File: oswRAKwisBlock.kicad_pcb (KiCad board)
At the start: 4 copper layers, 33.8 x 46 mm, 64 parts, among them J1 WisBlock, J2 0524352471, J4 10114830-10102LF, J5 USB micro, Q1 SI1308EDL-T1-GE3, U1 MCP73811T-420I/OT, U2 MAX2769B, U3 MAX8510EXK29+T, U4 MAX8510EXK29+T, Y1 TXETCDSANF-16.368000

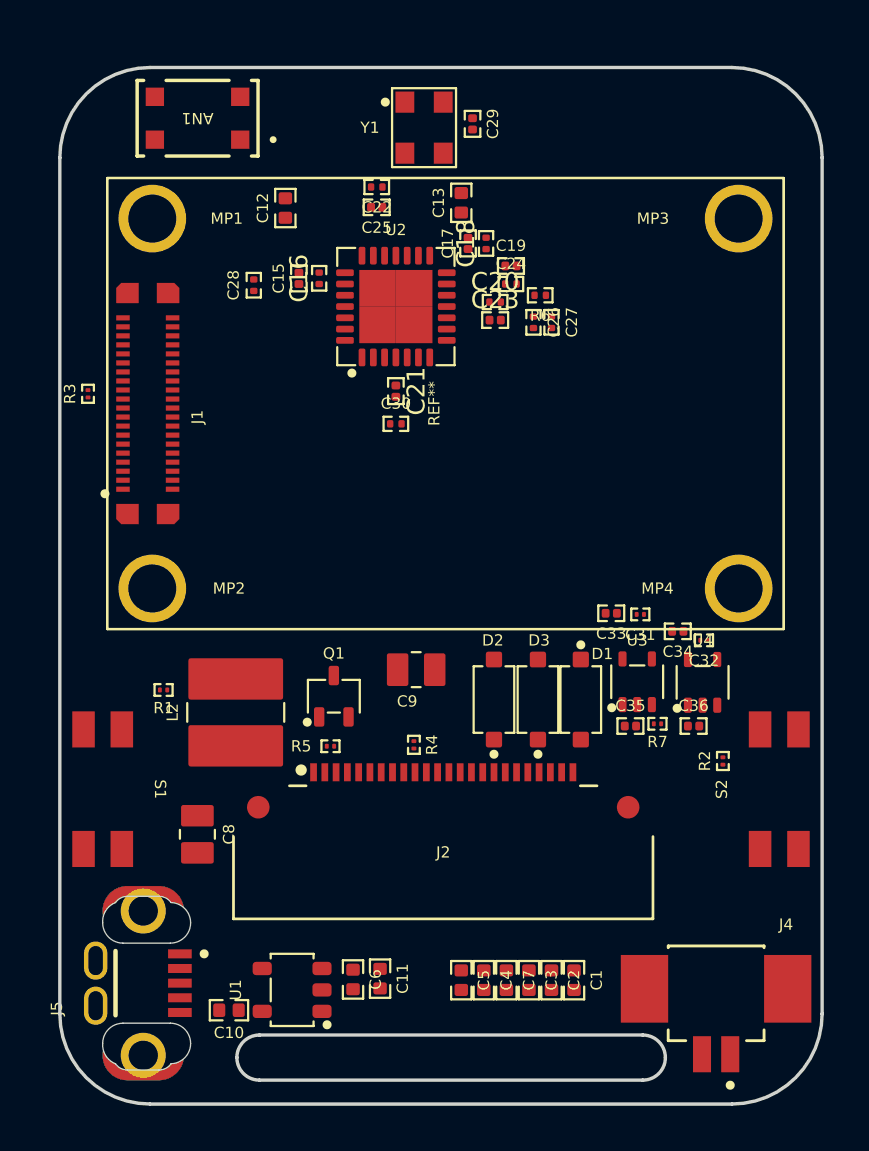
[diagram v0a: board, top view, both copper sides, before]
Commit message: starting to lay the board out.
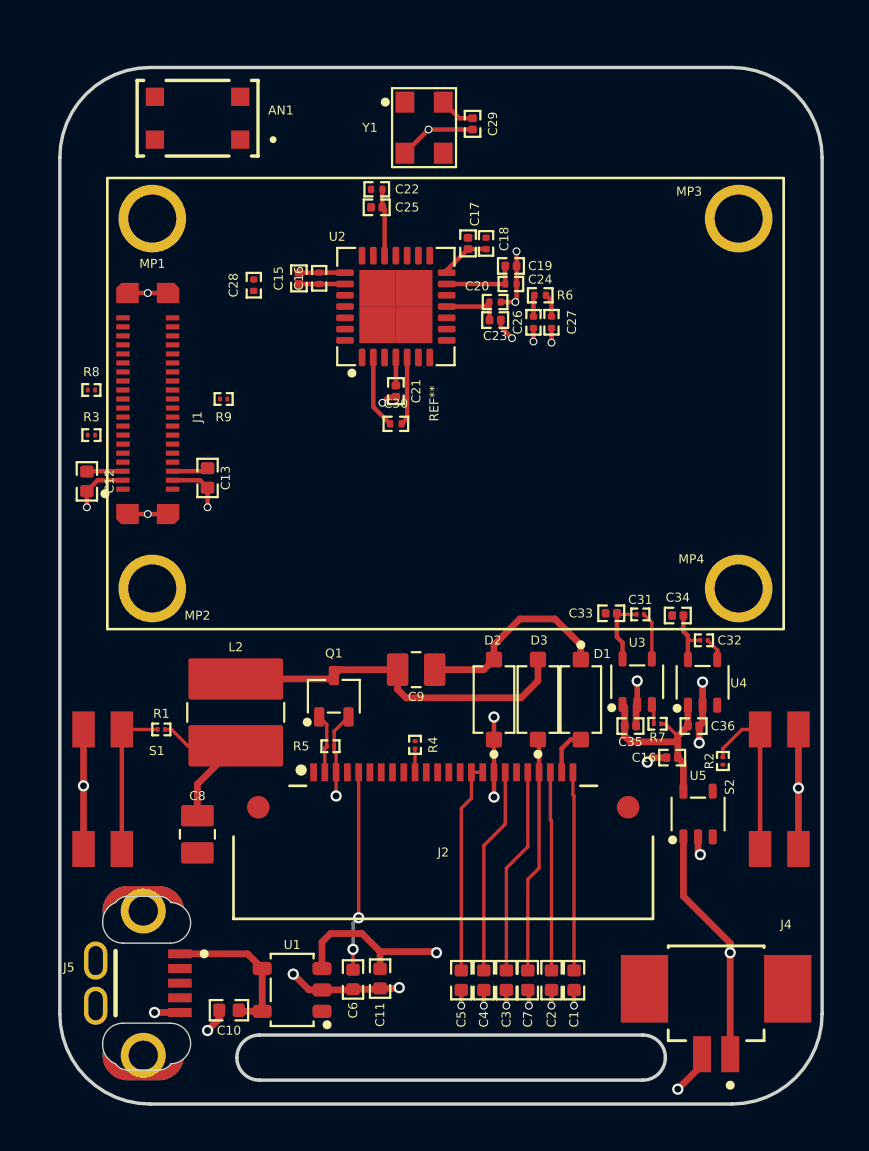
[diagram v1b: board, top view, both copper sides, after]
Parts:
- added C16: 1uF, AllardChip:CAPC60X30X39L17L, F.Cu at (147.0, 130.6)
- added R8: 10k, AllardChip:RESC40X20X15L10L, F.Cu at (121.2, 114.3)
- added R9: 10k, AllardChip:RESC40X20X15L10L, F.Cu at (127.1, 114.7)
- added U5: MIC5365-3.0YC5-TR, AllardSOT:SOT23-5P65_210X110L33X22L, F.Cu at (148.2, 133.1)
- moved C13 16.6 mm to (126.4, 118.2), turned to -90 degrees
- moved C12 15.0 mm to (121.0, 118.3), turned to -90 degrees
- moved R3 1.84 mm to (121.2, 116.3), turned to 0 degrees
- moved R1 1.75 mm to (124.3, 129.3)
- moved C3 1.00 mm to (139.7, 140.5)
- moved C7 0.95 mm to (140.6, 140.5)
- moved C34 0.70 mm to (147.2, 124.3)
- moved C22 0.10 mm to (133.9, 105.4)
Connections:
- J1 pad 22: unconnected-(J1-AIN1-Pad22) -> /~{GPS_PWR_SHDN}
- J1 pad 23: unconnected-(J1-BOOT-Pad23) -> Net-(J1-BOOT)
- J1 pad 24: unconnected-(J1-IO7-Pad24) -> /~{GPS_SHDN}
- J1 pad 25: unconnected-(J1-SPI_CS-Pad25) -> /SS
- J1 pad 26: unconnected-(J1-SPI_CLK-Pad26) -> /SCLK
- J1 pad 27: unconnected-(J1-SPI_MISO-Pad27) -> /GPS_MISO
- J1 pad 28: unconnected-(J1-SPI_MOSI-Pad28) -> /MOSI
- J1 pad 29: unconnected-(J1-IO1-Pad29) -> /BUSY
- J1 pad 30: unconnected-(J1-IO2-Pad30) -> /BTN1
- J1 pad 31: unconnected-(J1-IO3-Pad31) -> /RES
- J1 pad 32: unconnected-(J1-IO4-Pad32) -> /BTN2
- J1 pad 37: unconnected-(J1-IO5-Pad37) -> /~{GPS_IDLE}
- J1 pad 38: unconnected-(J1-IO6-Pad38) -> /~{GPS_CS}
- J1 pad FS3: (no net) -> GND
- R7 pad 2: /gpsMod/~{GPS_PWR_SHDN} -> /~{GPS_PWR_SHDN}
- U2 pad 10: /gpsMod/~{GPS_CS} -> /~{GPS_CS}
- U2 pad 24: /gpsMod/~{GPS_IDLE} -> /~{GPS_IDLE}
- U2 pad 7: /gpsMod/~{GPS_SHDN} -> /~{GPS_SHDN}
- U2 pad 8: /gpsMod/GPS_MISO -> /GPS_MISO
- U2 pad 9: /gpsMod/GPS_SCLK -> /SCLK
- U3 pad 3: /gpsMod/~{GPS_PWR_SHDN} -> /~{GPS_PWR_SHDN}
- U4 pad 3: /gpsMod/~{GPS_PWR_SHDN} -> /~{GPS_PWR_SHDN}
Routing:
- net GND: track 0.00 -> 58.0 mm, vias 0 -> 32
- net Net-(U1-V_{BAT}): track 0.00 -> 31.0 mm, vias 0 -> 2
- net VDD: track 0.00 -> 28.9 mm
- net Net-(Q1-D): track 0.00 -> 15.9 mm
- net VDD_GPS_A: track 0.00 -> 12.5 mm
- net /PREVGH: track 0.00 -> 10.5 mm
- net VDD_GPS_B: track 0.00 -> 9.71 mm
- net Net-(J2-Pin_20): track 0.00 -> 9.18 mm
- net Net-(J2-Pin_18): track 0.00 -> 9.18 mm
- net Net-(D1-K): track 0.00 -> 8.92 mm
- net Net-(J2-Pin_5): track 0.00 -> 8.86 mm, vias 0 -> 2
- net Net-(J2-Pin_24): track 0.00 -> 8.81 mm
- net Net-(J2-Pin_22): track 0.00 -> 8.81 mm
- net /BTN2: track 0.00 -> 7.69 mm
- net /BTN1: track 0.00 -> 6.89 mm
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- added copper zone on In1.Cu, net GND

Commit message: Moving some stuff around.
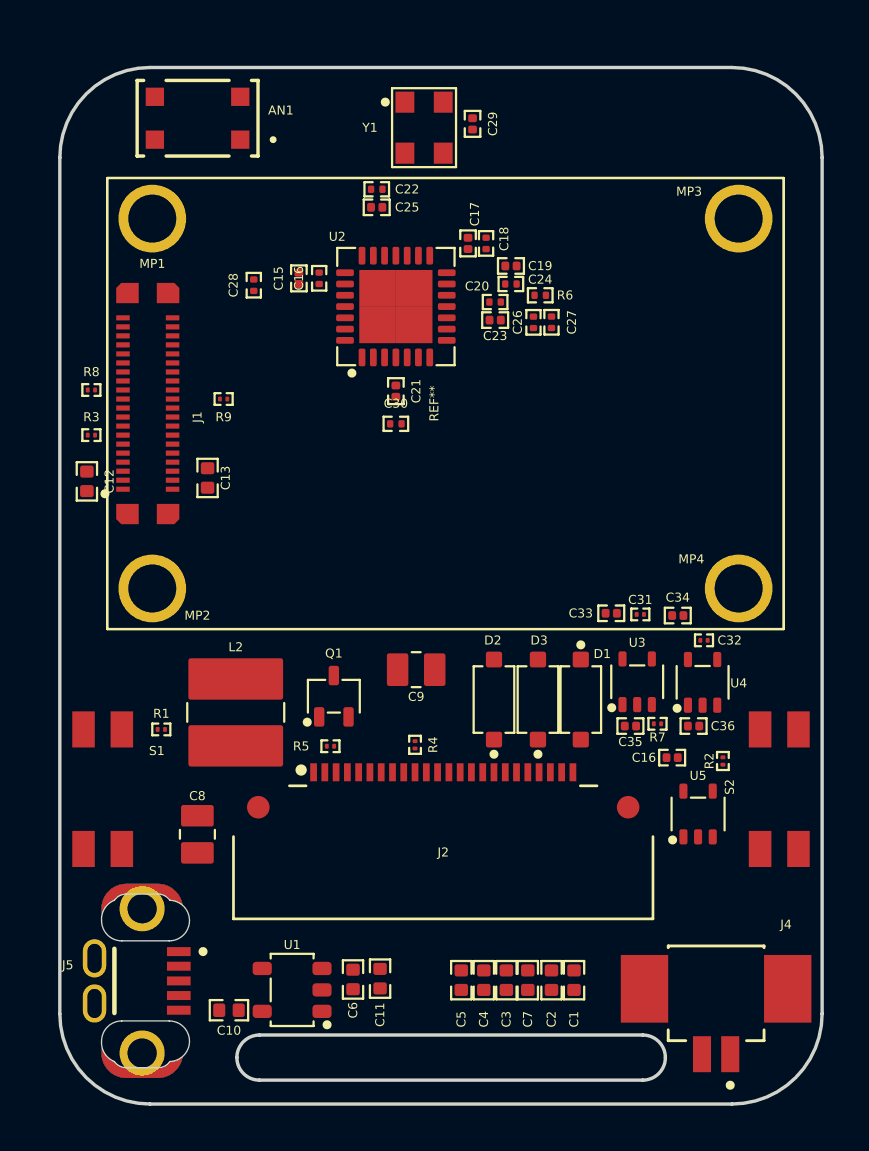
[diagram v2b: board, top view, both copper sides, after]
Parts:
- moved J5 0.11 mm to (123.5, 140.5)
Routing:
- net GND: track 58.0 -> 0.00 mm, vias 32 -> 0
- net Net-(U1-V_{BAT}): track 31.0 -> 0.00 mm, vias 2 -> 0
- net VDD: track 28.9 -> 0.00 mm
- net Net-(Q1-D): track 15.9 -> 0.00 mm
- net VDD_GPS_A: track 12.5 -> 0.00 mm
- net /PREVGH: track 10.5 -> 0.00 mm
- net VDD_GPS_B: track 9.71 -> 0.00 mm
- net Net-(J2-Pin_20): track 9.18 -> 0.00 mm
- net Net-(J2-Pin_18): track 9.18 -> 0.00 mm
- net Net-(D1-K): track 8.92 -> 0.00 mm
- net Net-(J2-Pin_5): track 8.86 -> 0.00 mm, vias 2 -> 0
- net Net-(J2-Pin_24): track 8.81 -> 0.00 mm
- net Net-(J2-Pin_22): track 8.81 -> 0.00 mm
- net /BTN2: track 7.69 -> 0.00 mm
- net /BTN1: track 6.89 -> 0.00 mm
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
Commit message: Moving some stuff around.
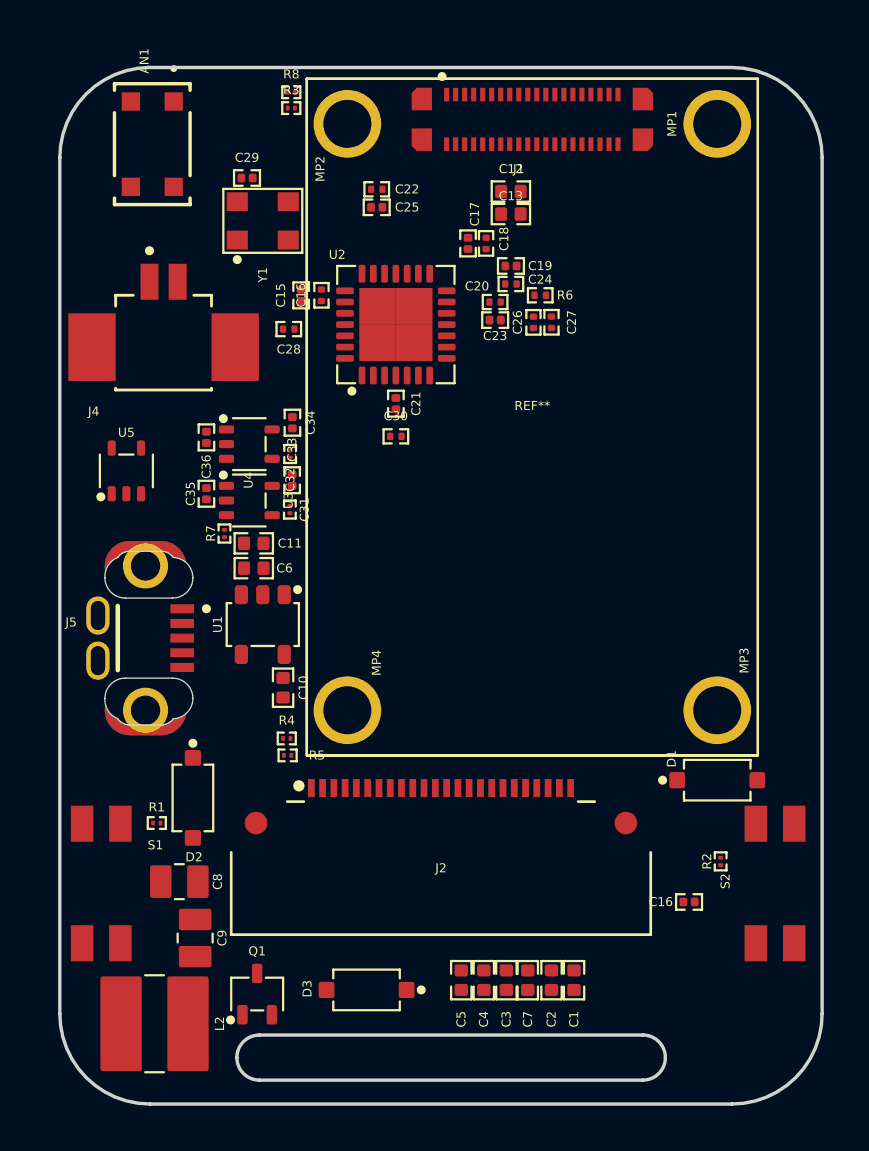
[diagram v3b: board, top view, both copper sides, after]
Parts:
- removed R9: 10k, AllardChip:RESC40X20X15L10L
- moved J4 37.8 mm to (124.5, 112.2), turned to 0 degrees
- moved U5 29.6 mm to (122.8, 117.9)
- moved MP1 25.4 mm to (149.0, 102.5), turned to -90 degrees
- moved C36 25.1 mm to (126.3, 116.4), turned to -90 degrees
- moved C12 22.8 mm to (139.8, 105.5), turned to 0 degrees
- moved U4 22.7 mm to (128.2, 116.7), turned to -90 degrees
- moved MP2 22.3 mm to (132.6, 102.5), turned to -90 degrees
- moved MP3 21.8 mm to (149.0, 128.5), turned to -90 degrees
- moved C35 21.4 mm to (126.3, 118.9), turned to -90 degrees
- moved J1 21.2 mm to (140.8, 102.3), turned to 0 degrees
- moved R7 21.0 mm to (127.2, 120.7), turned to 90 degrees
- moved C32 20.1 mm to (130.1, 117.1), turned to 90 degrees
- moved C11 20.1 mm to (128.4, 121.1), turned to 0 degrees
- moved C34 19.1 mm to (130.2, 115.8), turned to 90 degrees
- moved U3 19.0 mm to (128.2, 119.2), turned to -90 degrees
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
